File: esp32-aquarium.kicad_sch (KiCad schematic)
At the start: 3 parts, among them J1 12V IN, U1 esp32-wemos-d1-mini, U2 TSR 1-2433

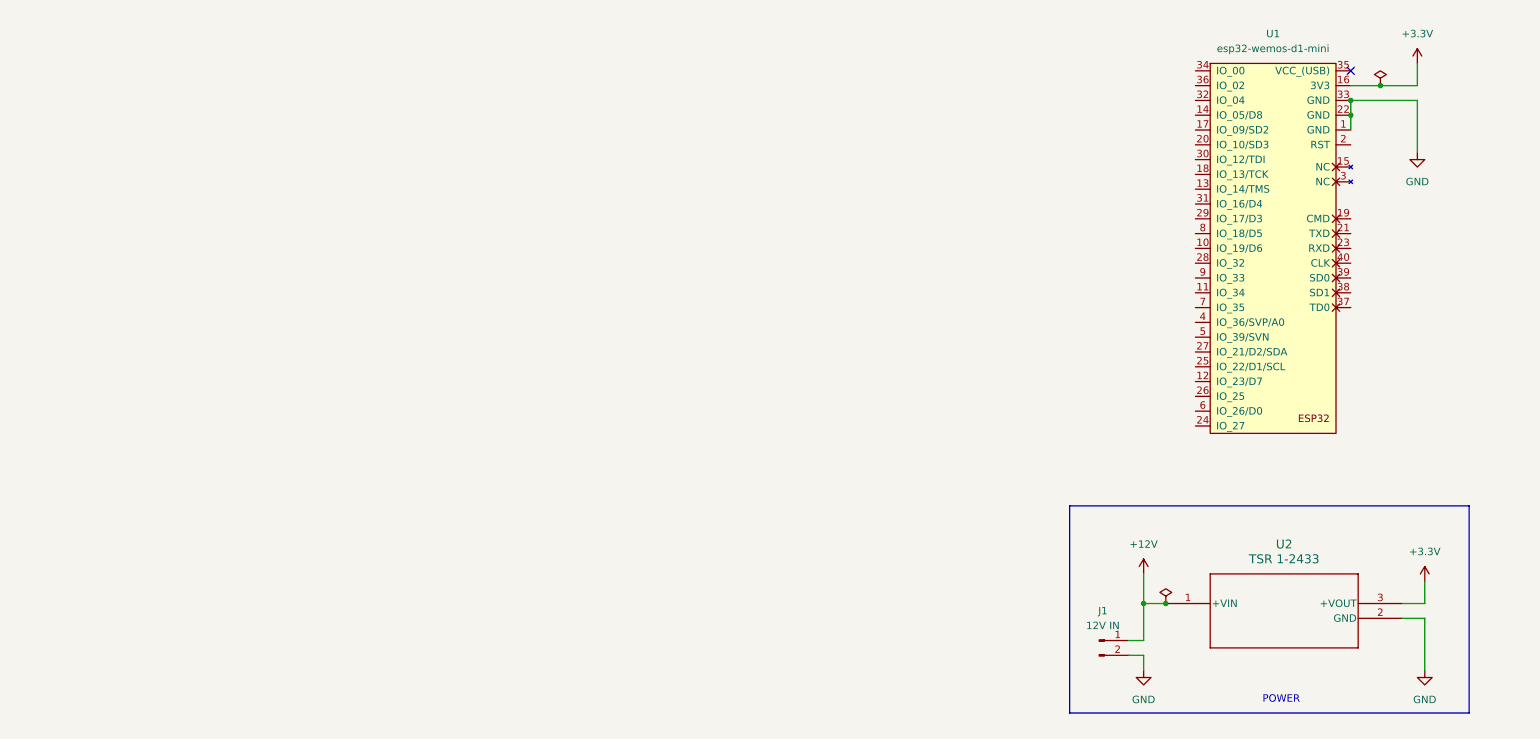
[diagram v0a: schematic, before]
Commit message: Start adding sensors
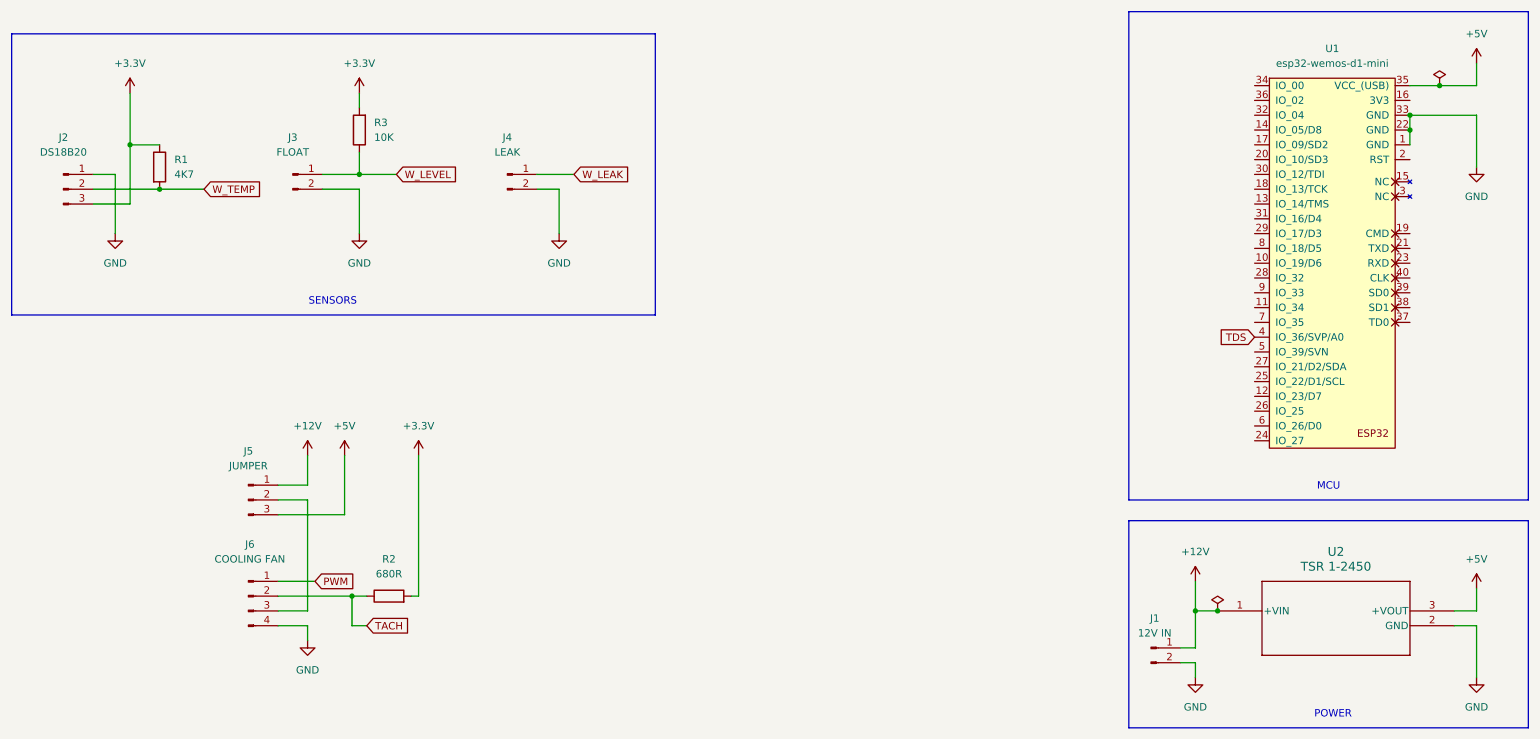
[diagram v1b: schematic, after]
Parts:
- removed U2: TSR 1-2433, TSR1-SINGLE_TRP, symbol 2025-10-06_03-42-38:TSR_1-2433
- added J2: DS18B20, Connector_JST:JST_XH_B3B-XH-A_1x03_P2.50mm_Vertical, symbol Connector:Conn_01x03_Pin
- added J3: FLOAT, Connector_JST:JST_XH_B2B-XH-A_1x02_P2.50mm_Vertical, symbol Connector:Conn_01x02_Pin
- added J4: LEAK, symbol Connector:Conn_01x02_Pin
- added J5: JUMPER, symbol Connector:Conn_01x03_Pin
- added J6: COOLING FAN, symbol Connector:Conn_01x04_Pin
- added R1: 4K7, Resistor_THT:R_Axial_DIN0204_L3.6mm_D1.6mm_P7.62mm_Horizontal, symbol Device:R
- added R2: 680R, symbol Device:R
- added R3: 10K, Resistor_THT:R_Axial_DIN0204_L3.6mm_D1.6mm_P7.62mm_Horizontal, symbol Device:R
- added U2: TSR 1-2450, TSR1-SINGLE_TRP, symbol 2026-02-07_07-09-34:TSR_1-2450
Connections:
- net +12V: now also J5.1 (Pin_1), U2.1 (+VIN)
- net +3.3V: now also J2.3 (Pin_3), R1.1, R2.2, R3.2; no longer U1.16 (3V3)
- net GND: now also J2.1 (Pin_1), J3.2 (Pin_2), J4.2 (Pin_2), J6.4 (Pin_4), U2.2 (GND)
- net +5V: now reaches U1.35 (VCC_(USB))
- net +5V: now also J5.3 (Pin_3), U2.3 (+VOUT)
- net TDS: now reaches U1.4 (IO_36/SVP/A0)
- new net: J5.2 (Pin_2), J6.3 (Pin_3)
- new net PWM: J6.1 (Pin_1)
- new net TACH: J6.2 (Pin_2), R2.1
- new net W_LEAK: J4.1 (Pin_1)
- new net W_LEVEL: J3.1 (Pin_1), R3.1
- new net W_TEMP: J2.2 (Pin_2), R1.2
- no-connect marks 1 -> 0
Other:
- note added: "MCU"
- note added: "SENSORS"
- moved on the sheet: J1, U1
